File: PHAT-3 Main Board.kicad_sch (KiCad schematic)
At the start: 19 parts, among them K1 G5LE-1, P1 Power Terminal Block, P2 Power Terminal Block, P3 Power Terminal Block, P4 Power Terminal Block, U1 AHT21, U10 Logic Level Converter, U2 ESP32-S3 Dual-core SX1262, U3 BME280, U4 GY-521 MPU-6050, U5 LM2596, U6 GT-7U, U7 SCD41, U8 uCAM-III, U9 SD Card Reader

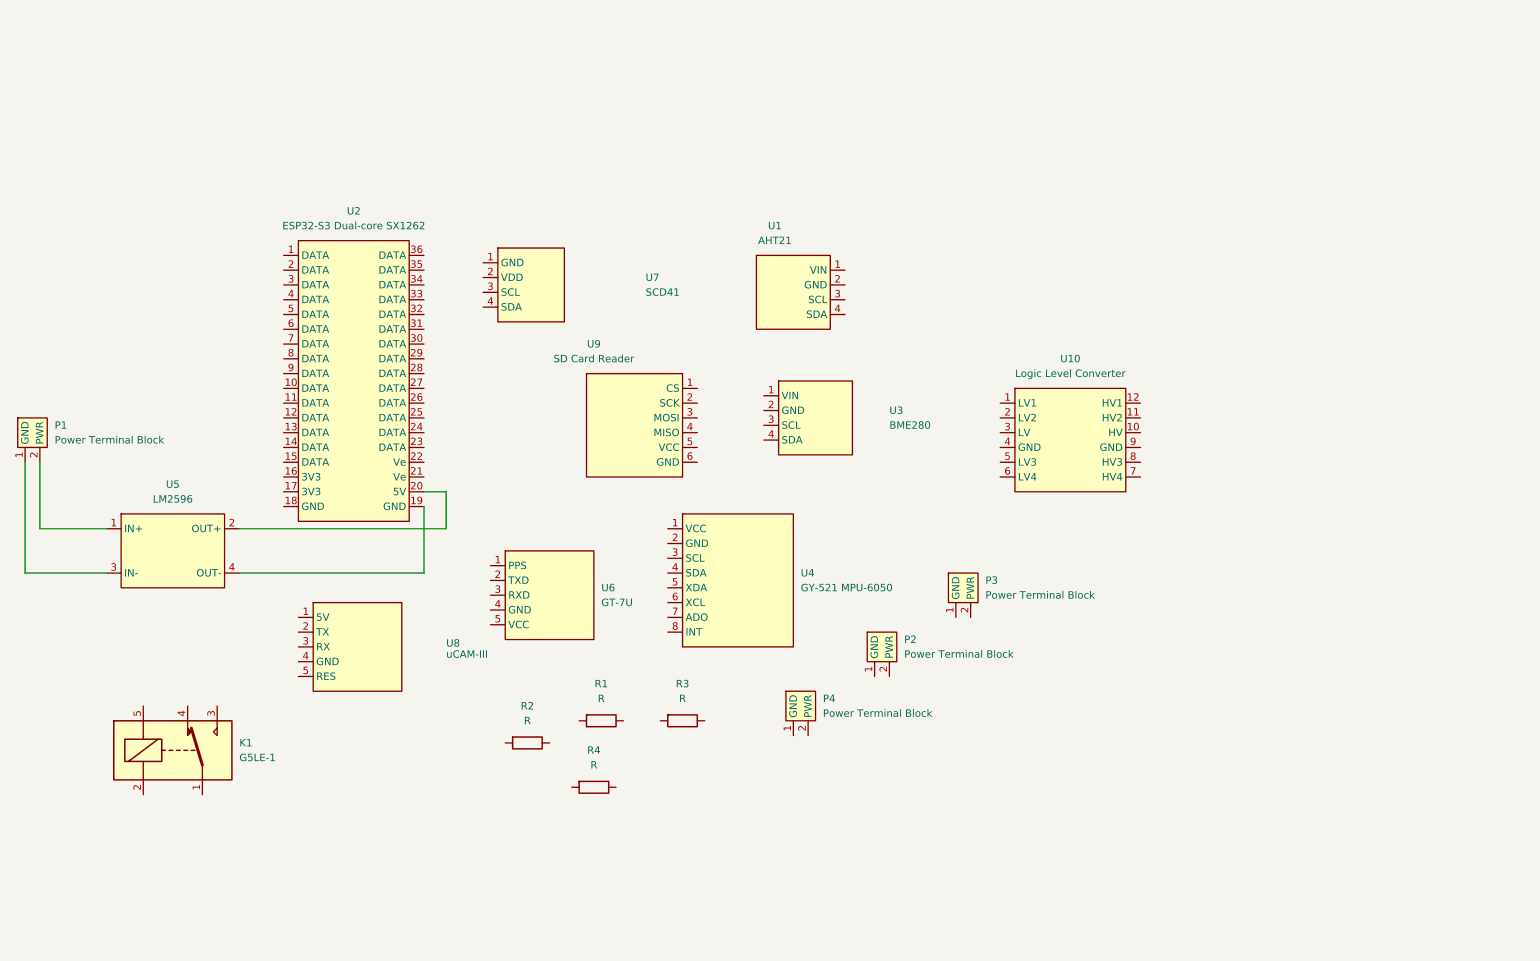
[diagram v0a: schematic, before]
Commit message: Tried Wiring Everything
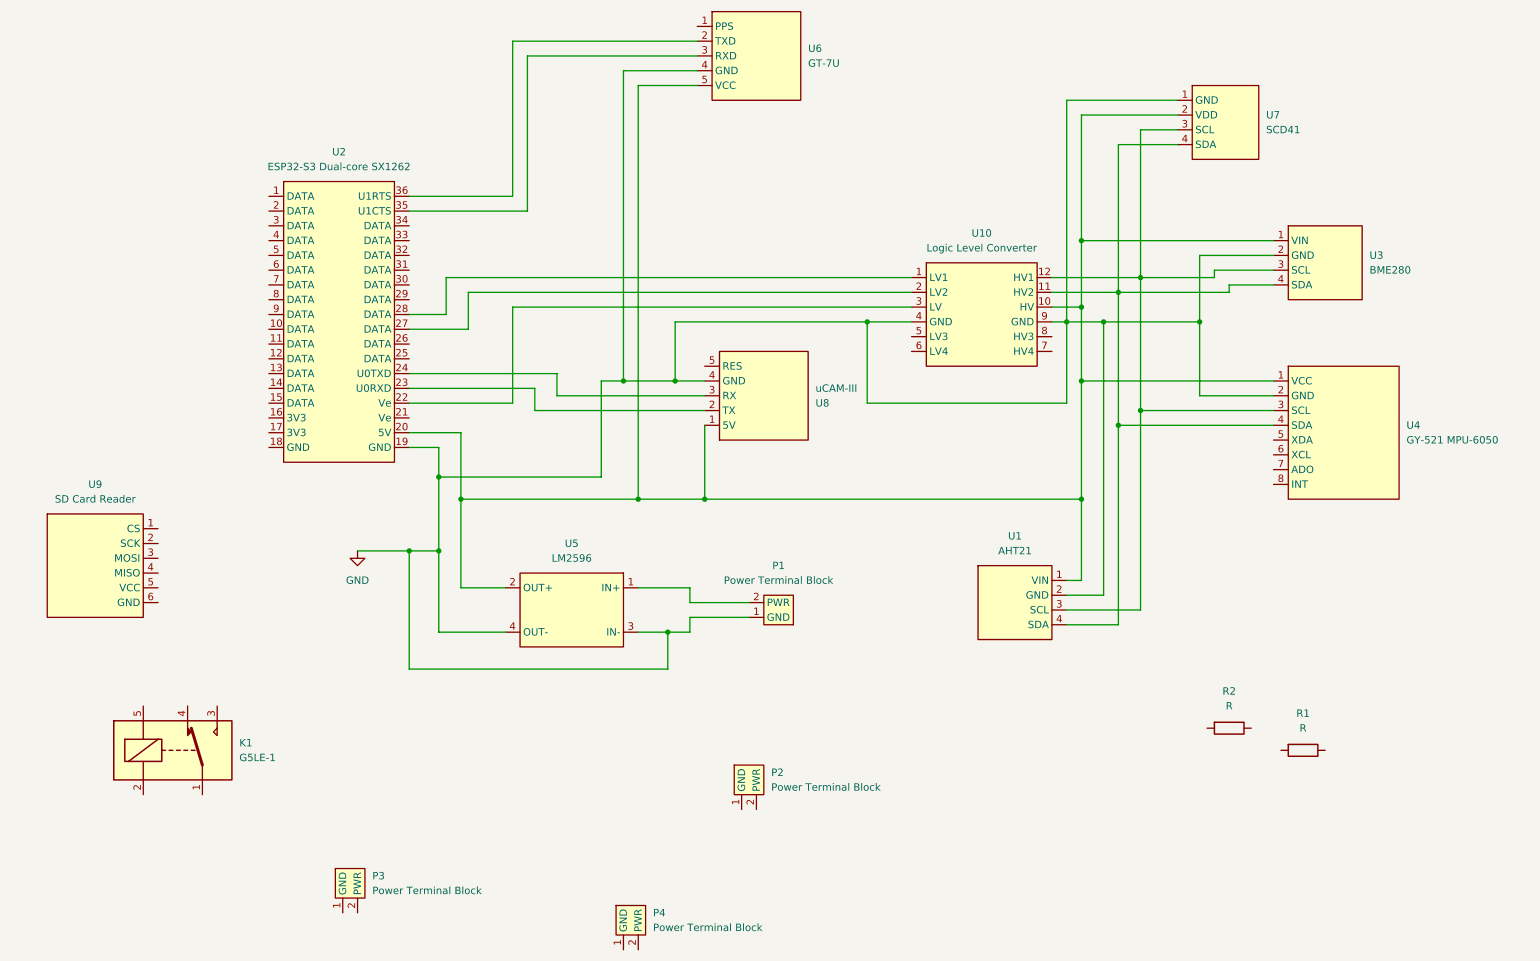
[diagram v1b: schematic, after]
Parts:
- removed R3, R4: R, Resistor_THT:R_Axial_DIN0207_L6.3mm_D2.5mm_P10.16mm_Horizontal, symbol Device:R
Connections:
- net at U6.2 (TXD): now also U2.36 (U1RTS)
- net at U6.3 (RXD): now also U2.35 (U1CTS)
- net GND: now reaches U6.4 (GND)
- net GND: now also P1.1 (GND), U1.2 (GND), U10.4 (GND), U10.9 (GND), U2.19 (GND), U3.2 (GND), U4.2 (GND), U5.3 (IN-), U5.4 (OUT-), U7.1 (GND), U8.4 (GND)
- net at U6.5 (VCC): now also U1.1 (VIN), U10.10 (HV), U2.20 (5V), U3.1 (VIN), U4.1 (VCC), U5.2 (OUT+), U7.2 (VDD), U8.1 (5V)
- net at U8.2 (TX): now also U2.23 (U0RXD)
- net at U8.3 (RX): now also U2.24 (U0TXD)
- net at U4.3 (SCL): now also U1.3 (SCL), U10.12 (HV1), U3.3 (SCL), U7.3 (SCL)
- net at U4.4 (SDA): now also U1.4 (SDA), U10.11 (HV2), U3.4 (SDA), U7.4 (SDA)
- net at U2.22 (Ve): now also U10.3 (LV)
- net at U2.27 (DATA): now also U10.2 (LV2)
- net at U2.28 (DATA): now also U10.1 (LV1)
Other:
- moved on the sheet: P1, P2, P3, P4, R2, U10, U2, U4, U5, U6
